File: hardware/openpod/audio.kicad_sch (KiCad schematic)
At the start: 29 parts, among them J1 SJ-43515TS-SMT-TR

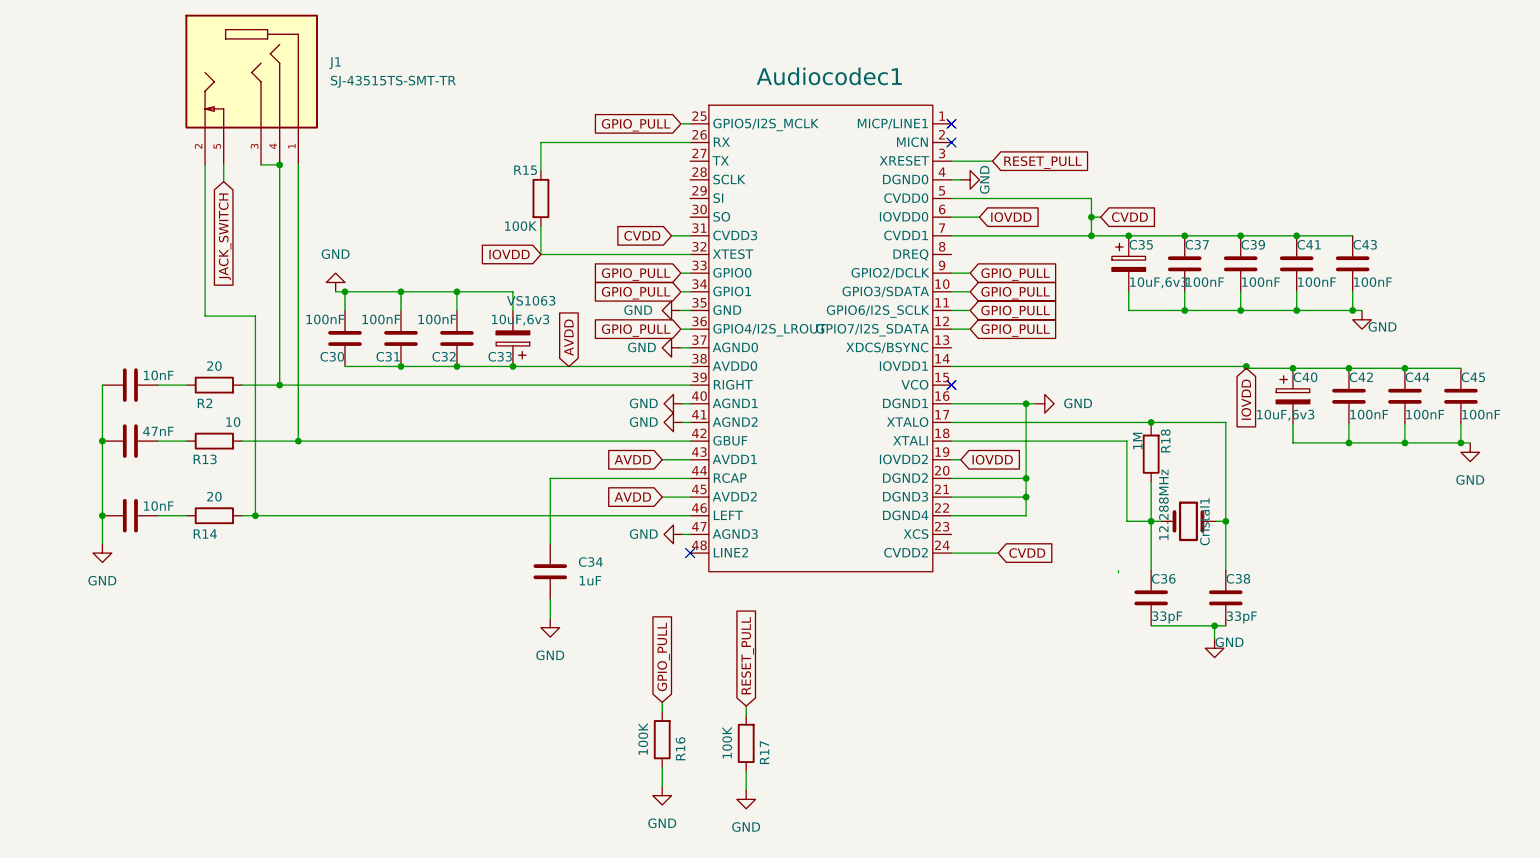
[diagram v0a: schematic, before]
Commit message: update power and audio
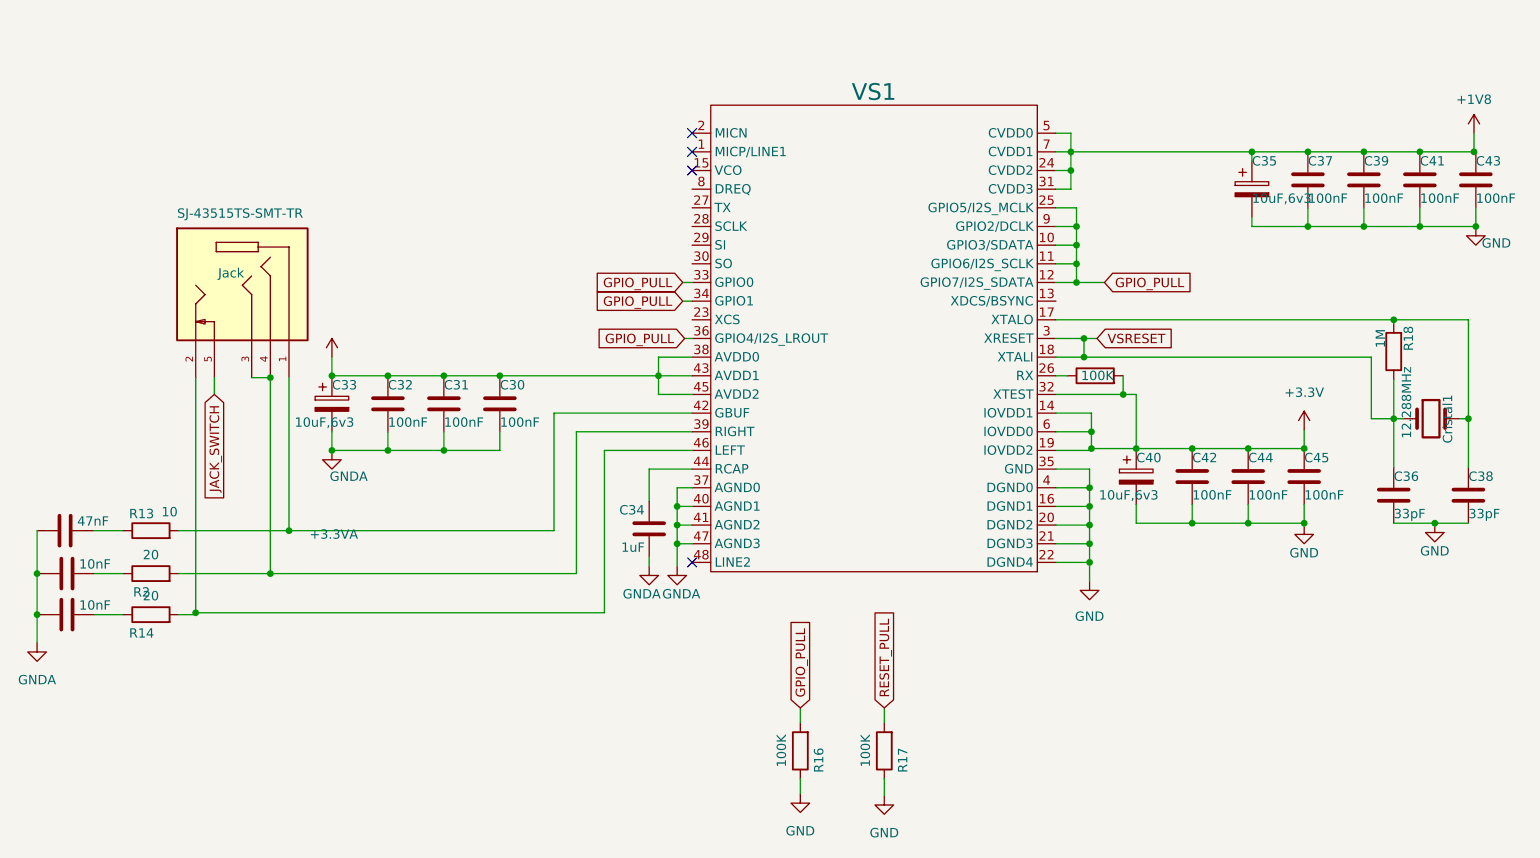
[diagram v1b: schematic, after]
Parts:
- removed Audiocodec1: VS1063, Package_QFP:LQFP-48-1EP_7x7mm_P0.5mm_EP3.6x3.6mm, symbol vs1063:vs1063
- removed R15: 100K, symbol Device:R
- added R1: 100K, symbol Device:R
- added VS1: ~, symbol openpod:vs1063
- renumbered J1 to Jack
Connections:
- net GND: now also VS1.16 (DGND1), VS1.20 (DGND2), VS1.21 (DGND3), VS1.22 (DGND4), VS1.35 (GND), VS1.4 (DGND0); no longer C29.1, C3.1, C30.2, C31.2, C32.2, C33.2, C34.2, C9.1
- net GPIO_PULL: now also VS1.10 (GPIO3/SDATA), VS1.11 (GPIO6/I2S_SCLK), VS1.12 (GPIO7/I2S_SDATA), VS1.25 (GPIO5/I2S_MCLK), VS1.33 (GPIO0), VS1.34 (GPIO1), VS1.36 (GPIO4/I2S_LROUT), VS1.9 (GPIO2/DCLK)
- net at C34.1: now also VS1.44 (RCAP)
- net at Jack.1, R13.2: now also VS1.42 (GBUF)
- net at Jack.2, R14.2: now also VS1.46 (LEFT)
- net at Jack.3, Jack.4, R2.2: now also VS1.39 (RIGHT)
- net VSRESET: now reaches C36.1, Cristal1.1, R18.1
- net VSRESET: now also VS1.18 (XTALI), VS1.3 (XRESET)
- net at C38.1, Cristal1.2, R18.2: now also VS1.17 (XTALO)
- net AVDD renamed +3.3VA
- net +3.3VA: now also VS1.38 (AVDD0), VS1.43 (AVDD1), VS1.45 (AVDD2)
- net CVDD renamed +1V8
- net +1V8: now also VS1.24 (CVDD2), VS1.31 (CVDD3), VS1.5 (CVDD0), VS1.7 (CVDD1)
- net IOVDD renamed +3.3V
- net +3.3V: now also R1.2, VS1.14 (IOVDD1), VS1.19 (IOVDD2), VS1.32 (XTEST), VS1.6 (IOVDD0)
- new net: R1.1, VS1.26 (RX)
- new net GNDA: C29.1, C3.1, C30.2, C31.2, C32.2, C33.2, C34.2, C9.1, VS1.37 (AGND0), VS1.40 (AGND1), VS1.41 (AGND2), VS1.47 (AGND3)
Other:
- moved on the sheet: C30, C31, C32, C33, C34, C35, C36, C37, C38, C39, C40, C41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
